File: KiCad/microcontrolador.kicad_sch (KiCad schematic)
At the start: 10 parts, among them J2 DE9_Pins_MountingHoles, U7 PIC24HJ128GP502-I_SO, Y1 8MHz

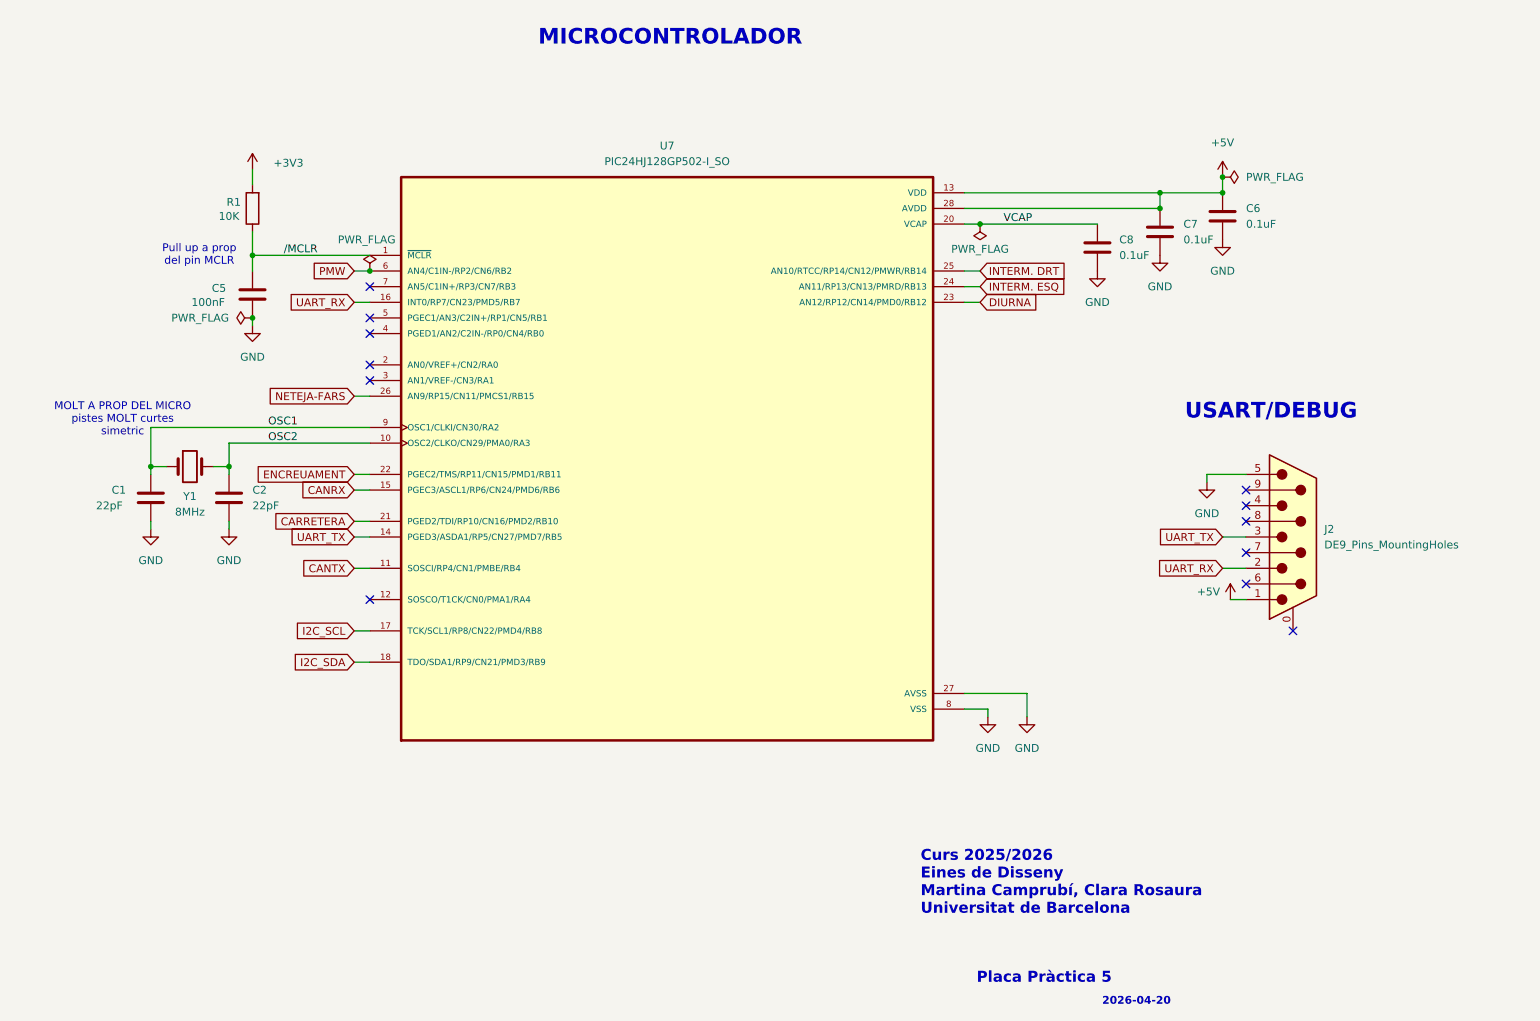
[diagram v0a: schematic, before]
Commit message: modificacions cadlab
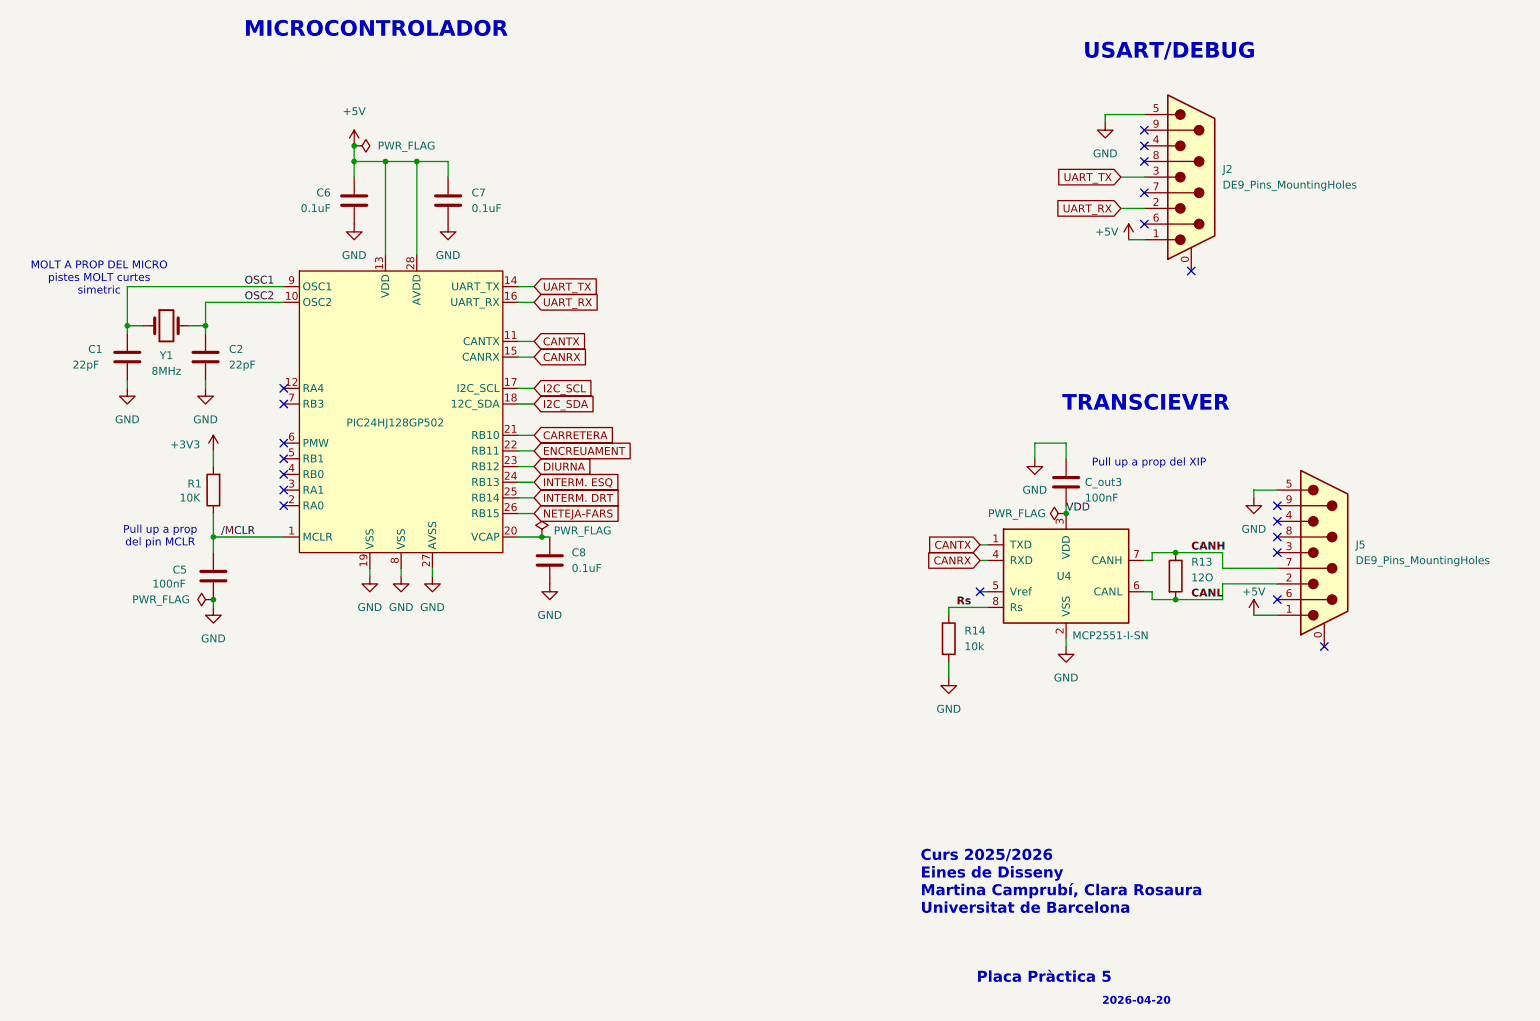
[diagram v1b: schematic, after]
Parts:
- removed U7: PIC24HJ128GP502-I_SO, footprints:SOIC127P1030X265-28N, symbol PIC24HJ128GP502-I_SO:PIC24HJ128GP502-I_SO
- added C_out3: 100nF, Capacitor_SMD:C_0805_2012Metric_Pad1.18x1.45mm_HandSolder, symbol Device:C
- added J5: DE9_Pins_MountingHoles, Connector_Dsub:DSUB-9_Pins_Horizontal_P2.77x2.84mm_EdgePinOffset4.94mm_Housed_MountingHolesOffset4.94mm, symbol Connector:DE9_Pins_MountingHoles
- added R13: 12O, Resistor_SMD:R_0805_2012Metric_Pad1.20x1.40mm_HandSolder, symbol Device:R
- added R14: 10k, Resistor_SMD:R_0805_2012Metric_Pad1.20x1.40mm_HandSolder, symbol Device:R
- added U2: ~, symbol PROJECTE_LLUMS:PIC24HJ128GP502
- added U4: MCP2551-I-SN, Package_SO:SOIC-8_3.9x4.9mm_P1.27mm, symbol Interface_CAN_LIN:MCP2551-I-SN
- added U7: PIC24HJ128GP502, projecte_llums:SOIC127P1030X265-28N, symbol PROJECTE_LLUMS:PIC24HJ128GP502
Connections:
- net +5V: now also J5.1, U7.13 (VDD), U7.28 (AVDD)
- net CANRX: now also U4.4 (RXD), U7.15 (CANRX)
- net CANTX: now also U4.1 (TXD), U7.11 (CANTX)
- net CARRETERA: now also U7.21 (RB10)
- net DIURNA: now also U7.23 (RB12)
- net ENCREUAMENT: now also U7.22 (RB11)
- net GND: now also C_out3.1, J5.5, R14.2, U4.2 (VSS), U7.19 (VSS), U7.27 (AVSS), U7.8 (VSS)
- net I2C_SCL: now also U7.17 (I2C_SCL)
- net I2C_SDA: now also U7.18 (12C_SDA)
- net INTERM. DRT: now also U7.25 (RB14)
- net INTERM. ESQ: now also U7.24 (RB13)
- net NETEJA-FARS: now also U7.26 (RB15)
- net OSC1: now also U7.9 (OSC1)
- net OSC2: now also U7.10 (OSC2)
- net UART_RX: now also U7.16 (UART_RX)
- net UART_TX: now also U7.14 (UART_TX)
- net /MCLR: now also U7.1 (MCLR)
- net VCAP: no longer names the net of C8.1
- net VCAP: now also U7.20 (VCAP)
- new net CANH: J5.7, R13.1, U4.7 (CANH)
- new net CANL: J5.2, R13.2, U4.6 (CANL)
- new net Rs: R14.1, U4.8 (Rs)
- new net VDD: C_out3.2, U4.3 (VDD)
- no-connect marks 12 -> 20
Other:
- note added: "Pull up a prop del XIP"
- note added: "TRANSCIEVER"
- moved on the sheet: C1, C2, C5, C6, C7, C8, J2, R1, Y1

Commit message: correccions Manel
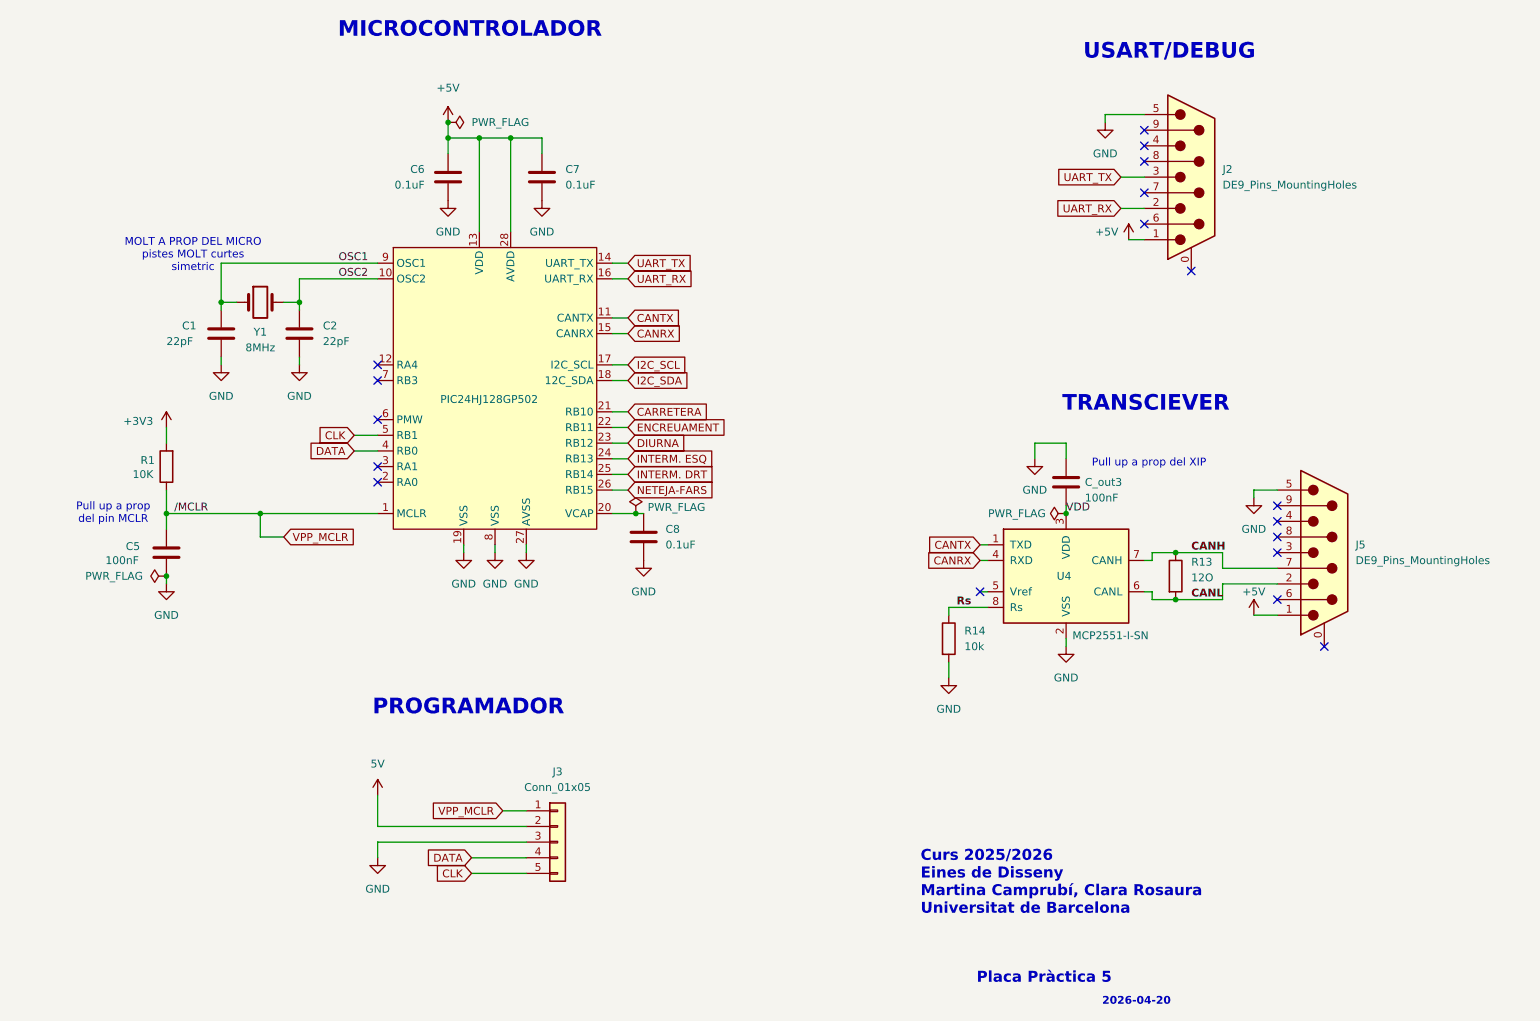
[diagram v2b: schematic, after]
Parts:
- added J3: Conn_01x05, Connector_PinHeader_2.54mm:PinHeader_1x05_P2.54mm_Vertical, symbol Connector_Generic:Conn_01x05
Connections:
- net GND: now also J3.3 (Pin_3)
- net DATA: now reaches U7.4 (RB0)
- net DATA: now also J3.4 (Pin_4)
- net CLK: now reaches U7.5 (RB1)
- net CLK: now also J3.5 (Pin_5)
- net /MCLR renamed VPP_MCLR
- net VPP_MCLR: now also J3.1 (Pin_1)
- new net 5V: J3.2 (Pin_2)
- no-connect marks 20 -> 18
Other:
- note added: "PROGRAMADOR"
- moved on the sheet: C1, C2, C5, C6, C7, C8, R1, Y1
